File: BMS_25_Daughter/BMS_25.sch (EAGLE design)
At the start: 178 parts, among them IC1 PBQ79656PAPTQ1, IC2 PBQ79656PAPTQ1, T1 PBHV8115X, 115, T2 PBHV8115X, 115

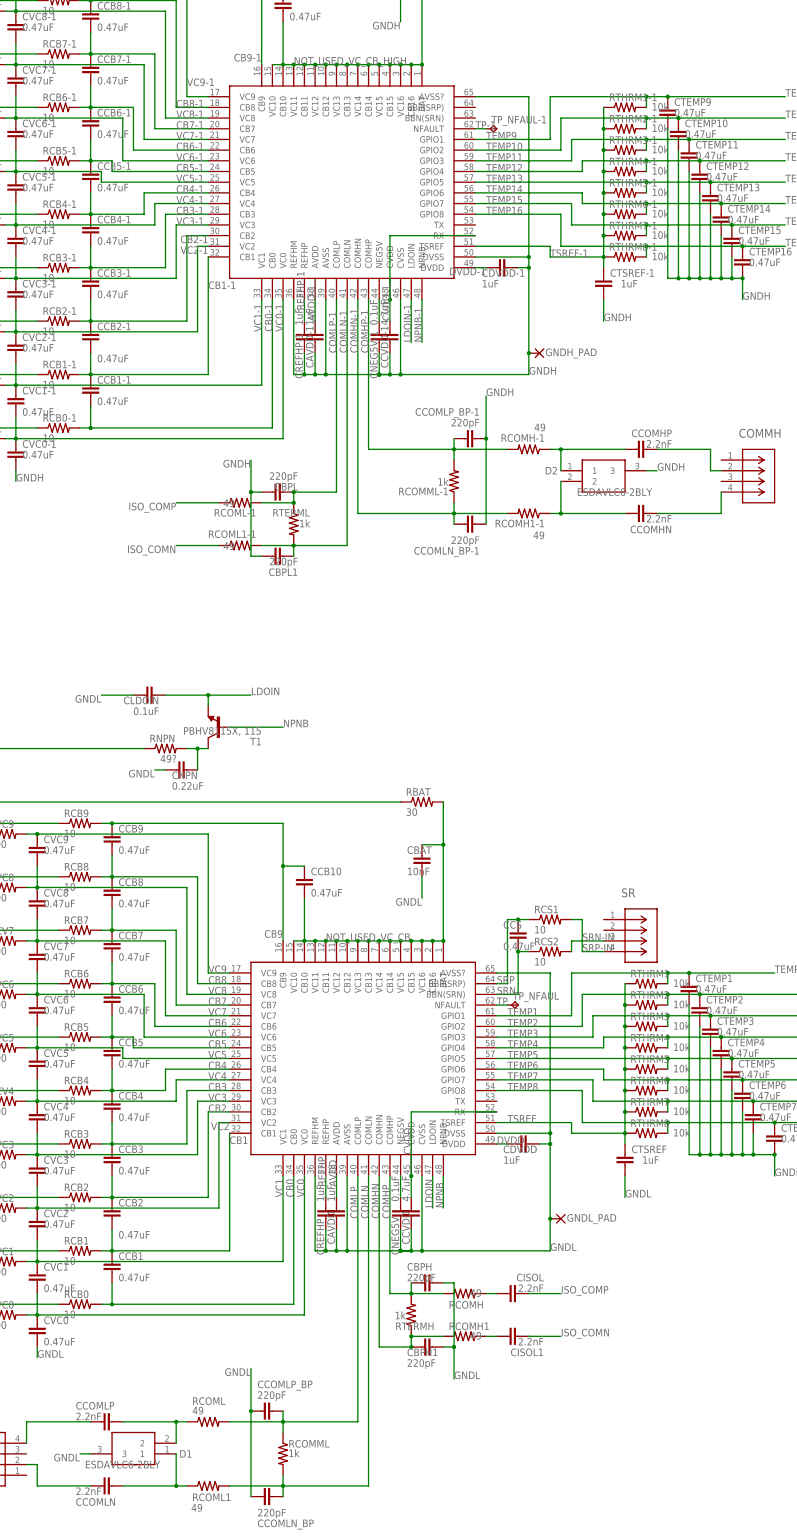
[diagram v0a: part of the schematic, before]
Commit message: Updated Change to daughteboard 14s for final manufacturing
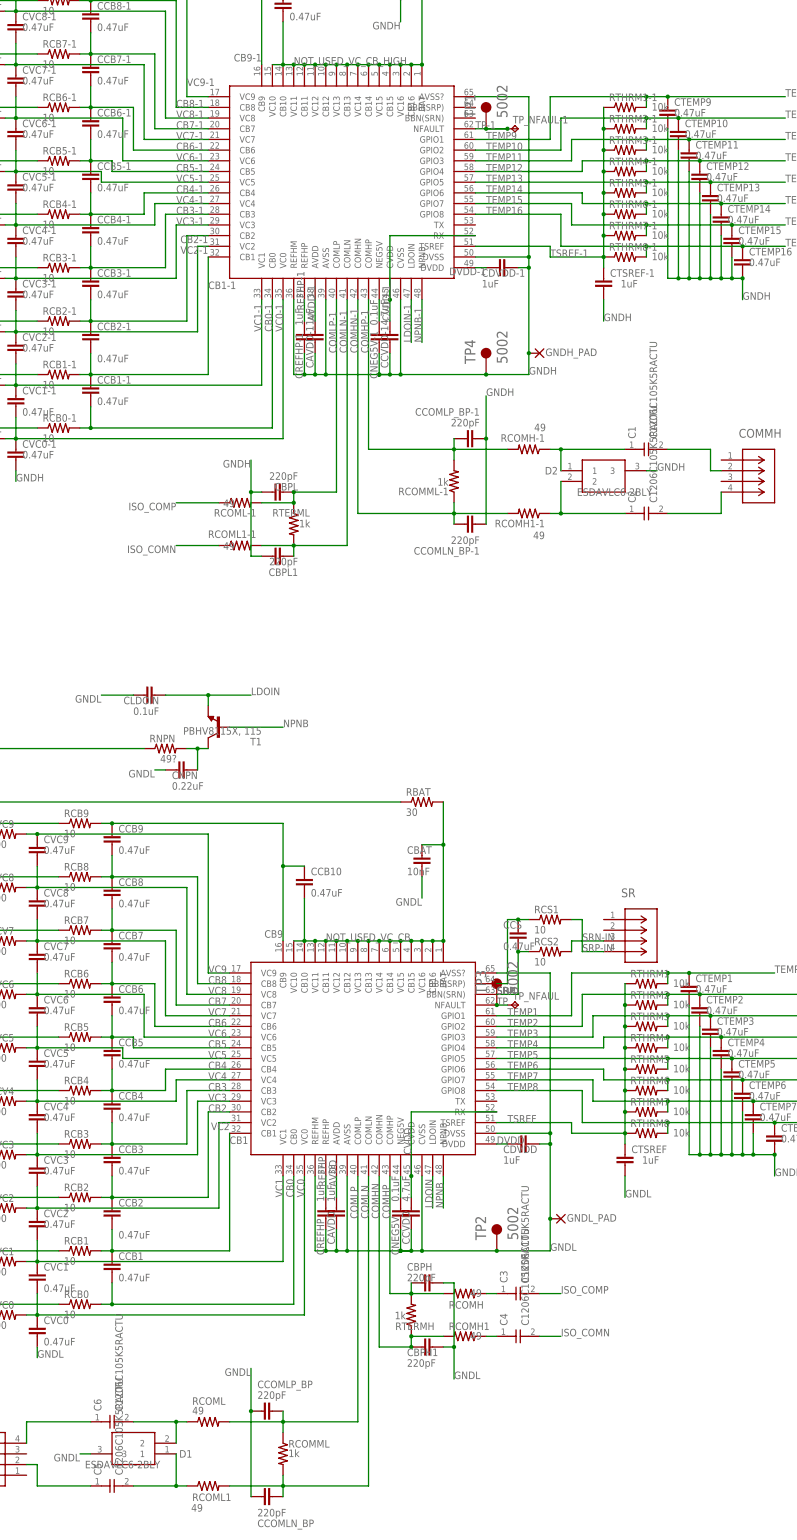
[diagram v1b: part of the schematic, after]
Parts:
- removed CCOMHN, CCOMHP, CCOMLN, CCOMLP, CISOL, CISOL1: 2.2nF, NFR23_v1.3:CAPACITORC0603
- added C1, C2, C3, C4, C5, C6: C1206C105K5RACTU, C1206C105K5RACTU:C1206C105K5RACTU
- added TP1, TP2, TP3, TP4: 5002, 5002:5002
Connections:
- net GNDH: now also TP4.TP
- net GNDL: now also TP2.TP
- net ISO_COMN: now also C4.B; no longer CISOL1.1
- net ISO_COMP: now also C3.B; no longer CISOL.1
- net N$101: now also C2.B; no longer CCOMHN.1
- net N$103: now also C5.A; no longer CCOMLN.1
- net N$104: now also C6.A; no longer CCOMLP.1
- net N$46: now also C3.A; no longer CISOL.2
- net N$47: now also C4.A; no longer CISOL1.2
- net N$50: now also C5.B; no longer CCOMLN.2
- net N$51: now also C6.B; no longer CCOMLP.2
- net N$97: now also C1.A; no longer CCOMHP.2
- net N$98: now also C2.A; no longer CCOMHN.2
- net N$99: now also C1.B; no longer CCOMHP.1
- net TP: now also TP3.TP
- net TP-1: now also TP1.TP
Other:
- moved on the sheet: TP_NFAUL-1
